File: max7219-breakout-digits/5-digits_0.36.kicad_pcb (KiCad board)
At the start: 2 copper layers, 53.5 x 15.5 mm, 6 parts, among them J1 Conn_02x08_Odd_Even, U1 HDSM-443B_7-Segment_2_Digit, U2 HDSM-443B_7-Segment_3_Digit

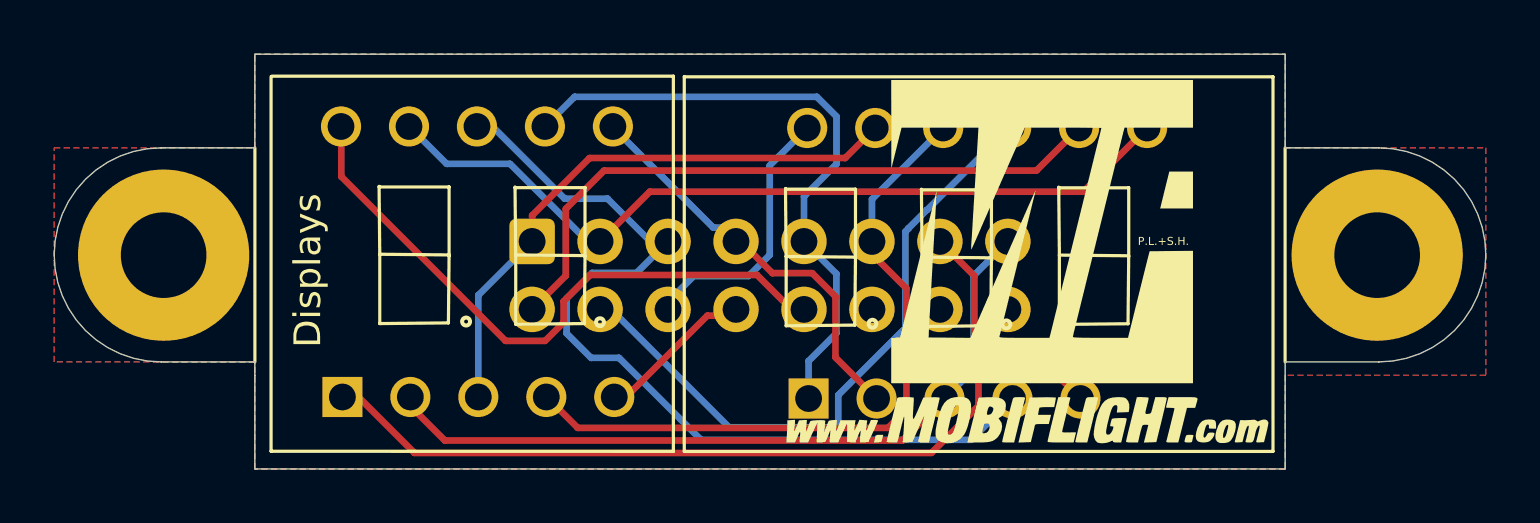
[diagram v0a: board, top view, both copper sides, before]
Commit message: upadate labels
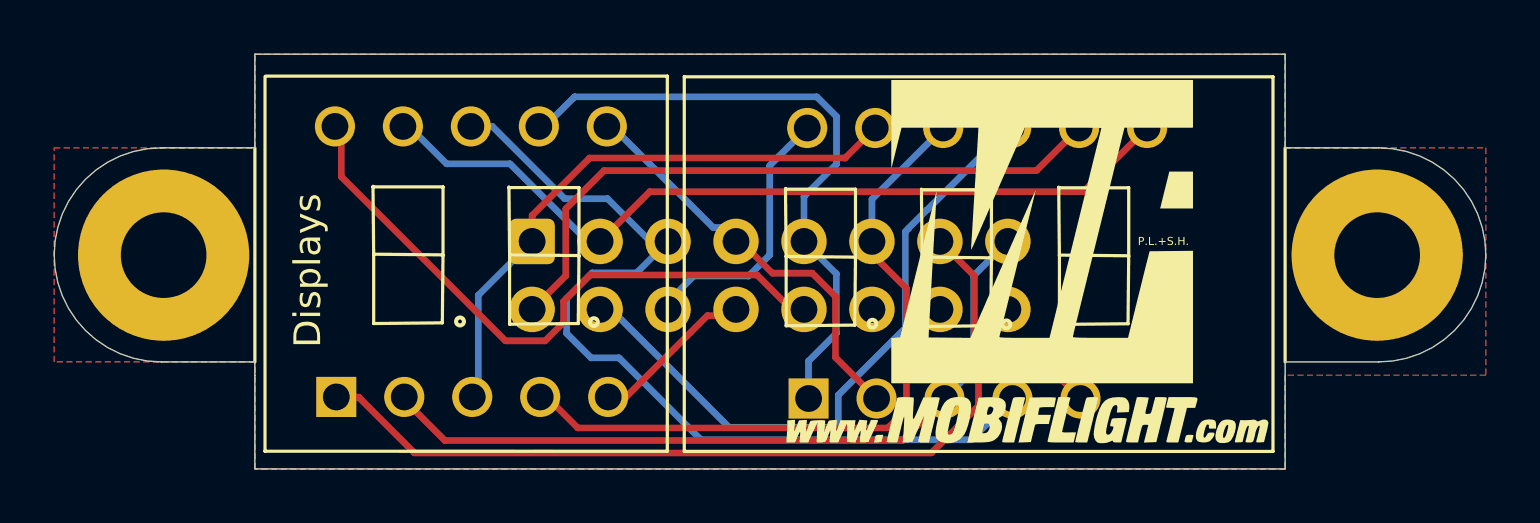
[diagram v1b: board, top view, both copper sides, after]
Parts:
- moved U1 0.23 mm to (102.0, 47.7)
